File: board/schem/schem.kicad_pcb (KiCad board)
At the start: 2 copper layers, 133 x 86 mm, 146 parts, among them J1 no_break, J10 no_hal, J11 break2, J12 impulse, J13 hal, J14 no_temp, J15 speed, J16 analog, J17 motor_tmp, J18 adc_red1, J19 adc_red2, J2 motor_out, J20 ON/OFF, J21 lamp, J3 test, J8 POWER_IN, J9 break1, Q1 BC817, Q2 BC807, Q3 BC817, Q4 BC817, Q5 BC807, Q6 BC817, Q7 BC817, Q8 BC807, Q9 BC817, SW1 SW_Push, SW2 SW_Push, T1 NTD5865NL, T2 FDD9507L, T3 NTD5865NL, T4 FDD9507L, T5 NTD5865NL, T6 FDD9507L, U1 CFPS-39-12M, U10 AP2138, U11 LD1117, U12 68u, U2 EP4CE6, U3 JTAG, U4 IS25LQ, U5 LF33CDT, U6 IS25LQ, U7 MPC3008, U8 A8498, U9 B350B

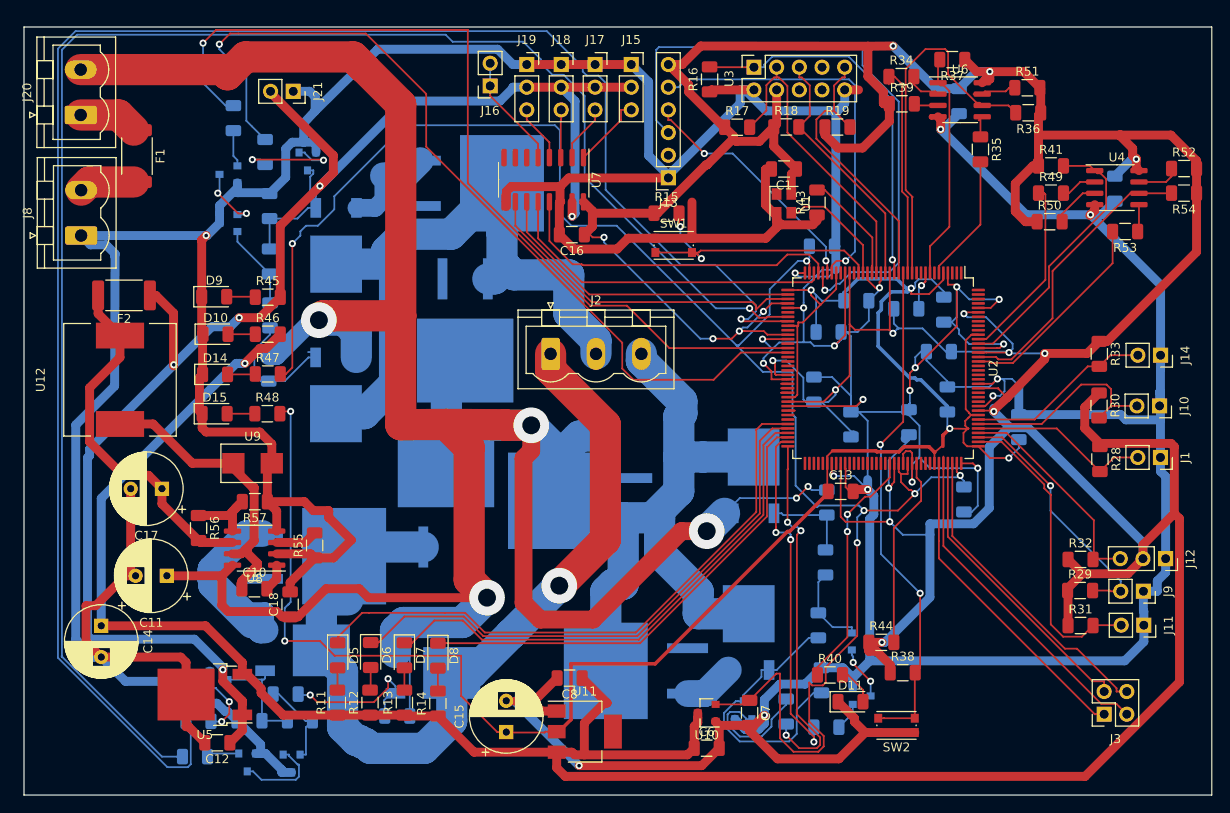
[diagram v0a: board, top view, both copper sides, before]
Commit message: recent  changes
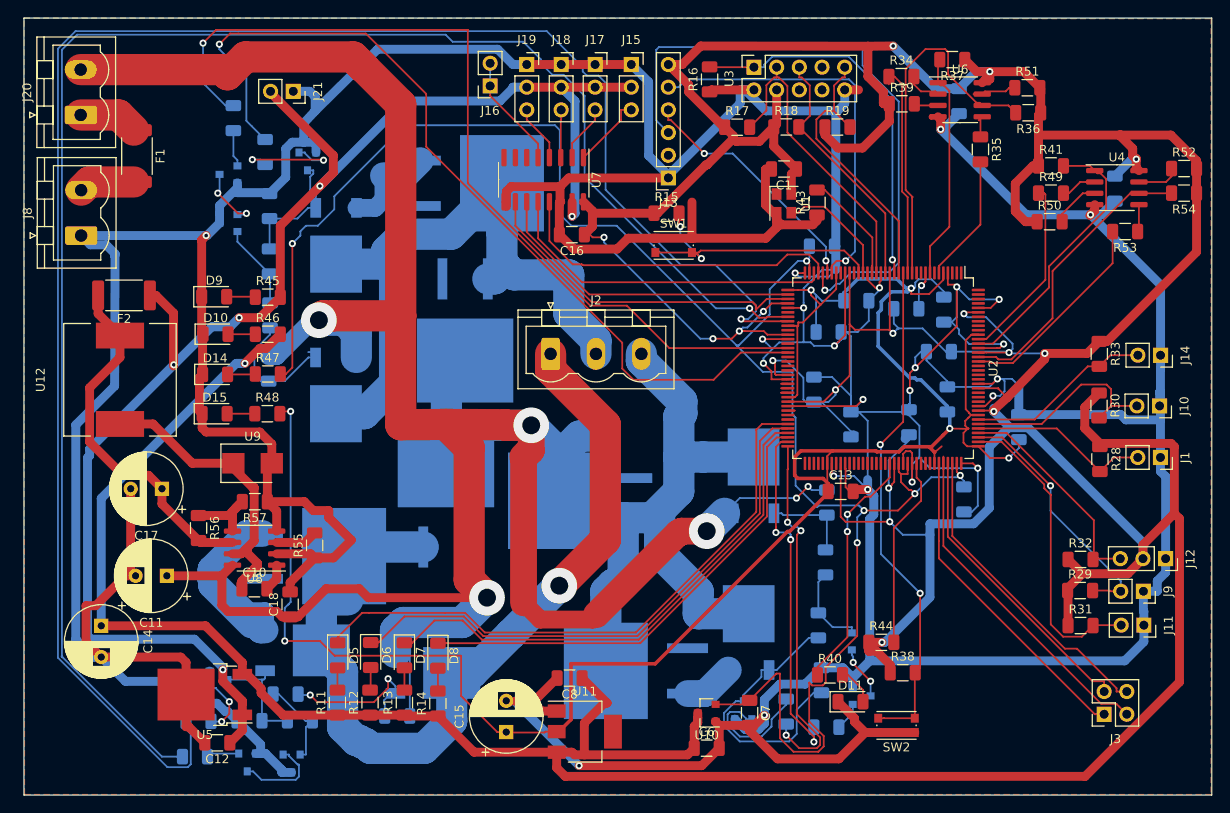
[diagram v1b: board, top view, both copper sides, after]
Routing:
- net +36V: track 302.0 -> 337.2 mm
- net +1V2: track 233.5 -> 245.8 mm
- added copper zone on B.Cu, net GND
- added copper zone on F.Cu, net GND
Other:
- board size 133 x 86 mm -> 133 x 87 mm
- net class energy_mid: trace_width 2 -> 3
